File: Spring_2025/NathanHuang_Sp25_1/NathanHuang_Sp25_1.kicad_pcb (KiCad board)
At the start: 2 copper layers, 13 parts, among them J1 Barrel_Jack, M1 Motor_Servo, M2 Motor_Servo, M3 Motor_Servo, M4 Motor_Servo, M5 Motor_Servo, M6 Motor_Servo, M7 Stepper_Motor_bipolar, U1 ESP32-DEVKITC-32UE, U2 LM2596_BUCK_CONVERTER

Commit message: PCB Changes
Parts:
- removed the J1 at (240.5, 53.5)
- removed the J1 at (274.5, 48.0)
- added J1: Barrel_Jack, Connector_BarrelJack:BarrelJack_SwitchcraftConxall_RAPC10U_Horizontal, F.Cu at (54.7, 41.5)
- moved C1 178.3 mm to (74.0, 41.0), turned to 180 degrees
- moved A1 171.6 mm to (57.2, 93.2), turned to 180 degrees
- moved M7 160.1 mm to (76.5, 86.0), turned to 180 degrees
- moved U2 156.0 mm to (123.1, 49.0), turned to 180 degrees
- moved U1 52.4 mm to (103.2, 95.9)
- moved M6 27.6 mm to (143.5, 119.5)
- moved M5 26.7 mm to (143.6, 110.5)
- moved M4 24.4 mm to (143.1, 100.0)
- moved M3 23.0 mm to (143.0, 89.5)
- moved M2 21.5 mm to (143.1, 76.5)
- moved M1 21.2 mm to (143.0, 64.0)
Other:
- board outline added: 139.5 x 109.5 mm
- board text added: "12 V Side"
- board text added: "7.2 V Side"

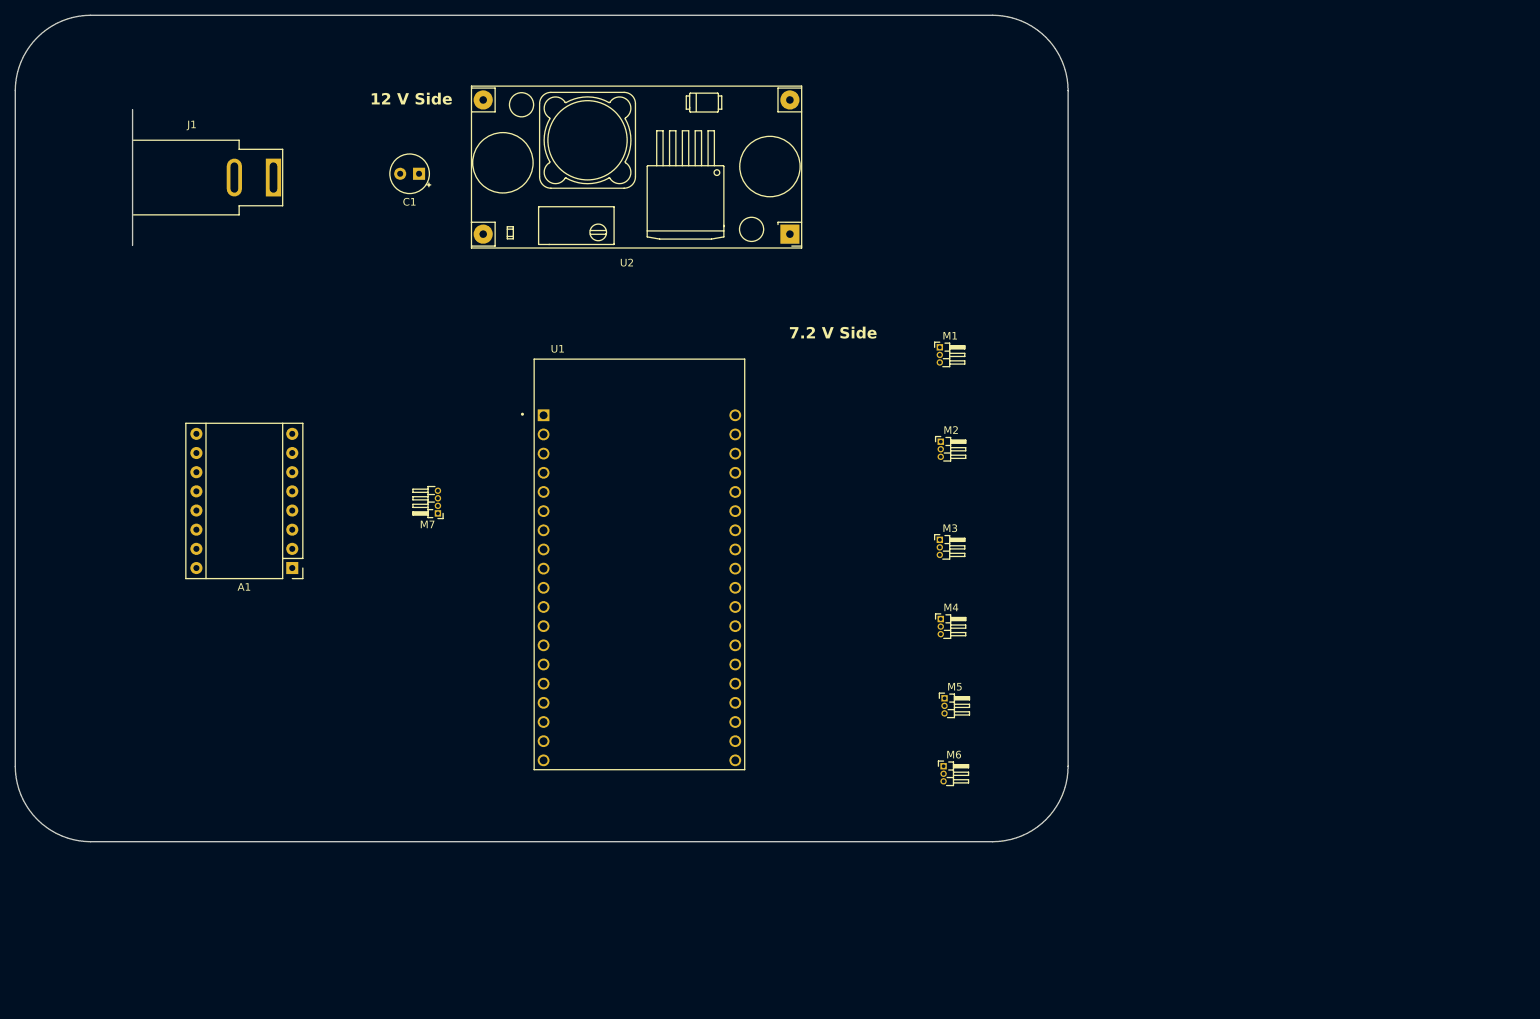
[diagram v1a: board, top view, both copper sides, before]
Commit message: Finished PCB, Ready for Print
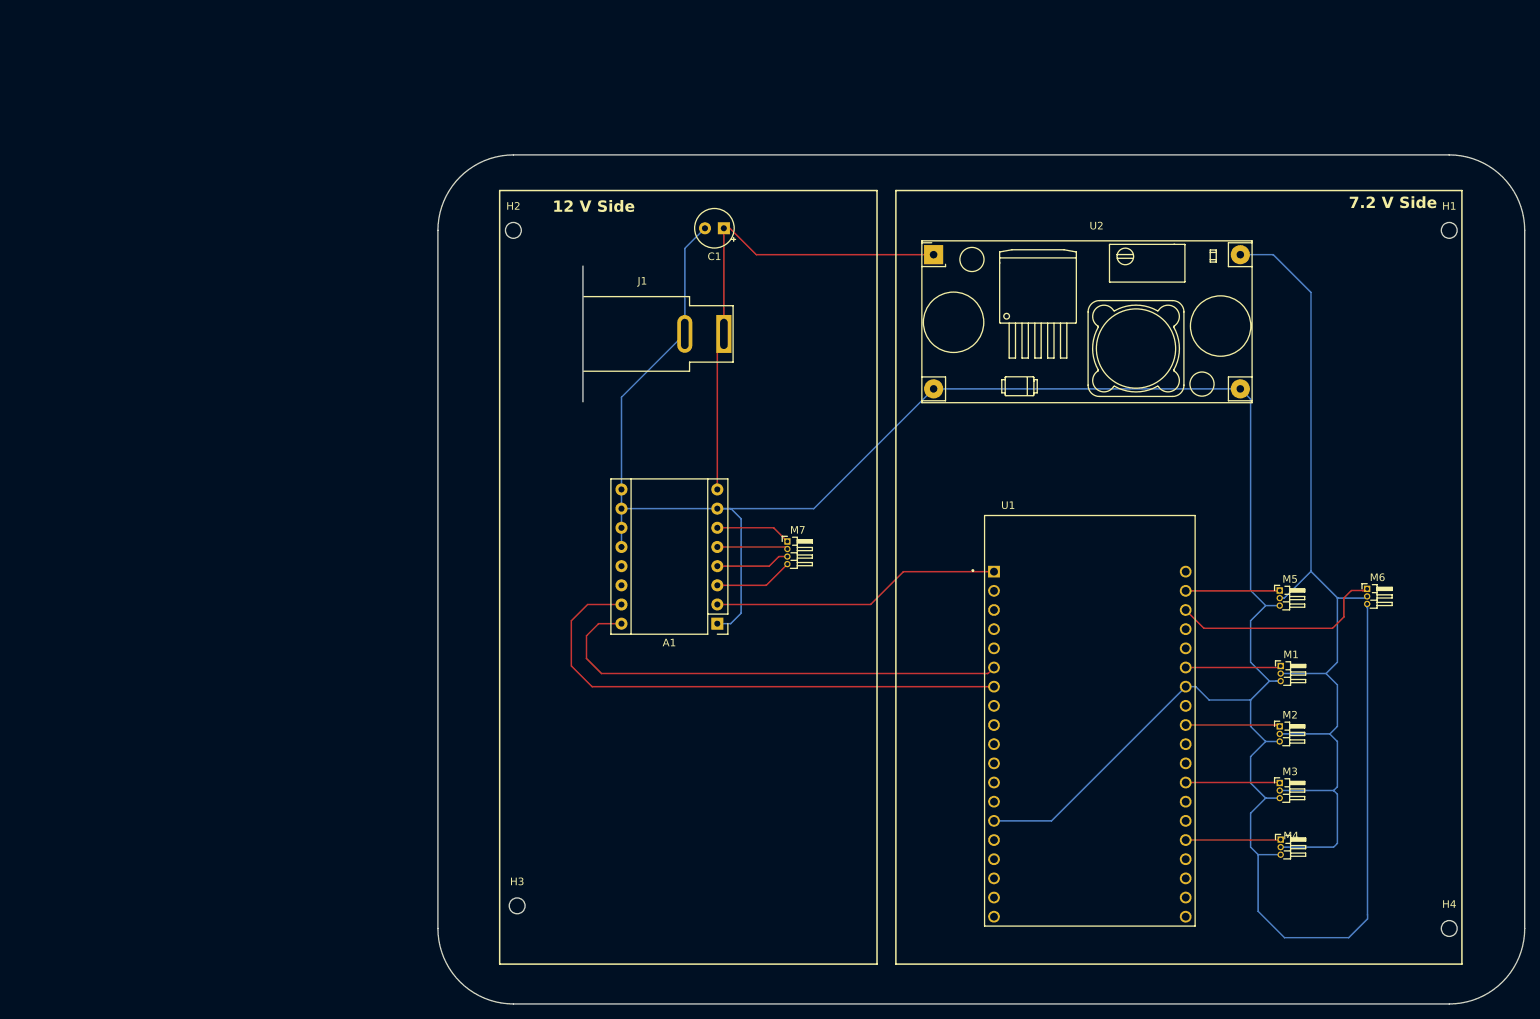
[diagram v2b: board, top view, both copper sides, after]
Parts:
- added H1: MountingHole, MountingHole:MountingHole_2.1mm, F.Cu at (210.5, 48.5)
- added H2: MountingHole, MountingHole:MountingHole_2.1mm, F.Cu at (86.5, 48.5)
- added H3: MountingHole, MountingHole:MountingHole_2.1mm, F.Cu at (87.0, 138.0)
- added H4: MountingHole, MountingHole:MountingHole_2.1mm, F.Cu at (210.5, 141.0)
- moved J1 63.2 mm to (114.4, 62.2)
- moved U1 63.2 mm to (162.9, 116.6)
- moved M1 61.8 mm to (188.2, 106.2)
- moved M6 60.8 mm to (199.6, 96.0)
- moved M2 58.7 mm to (188.0, 114.2)
- moved A1 56.8 mm to (113.5, 100.6)
- moved M3 55.4 mm to (188.0, 121.7)
- moved M4 53.7 mm to (188.2, 129.2)
- moved M5 46.7 mm to (188.0, 96.2)
- moved M7 46.5 mm to (122.8, 89.7), turned to 0 degrees
- moved C1 41.0 mm to (114.4, 48.2)
- moved U2 19.2 mm to (142.2, 51.7), turned to 0 degrees
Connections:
- A1 pad 2: +5V -> +3V3
- M7 pad 1: Net-(A1-1B) -> Net-(A1-2B)
- M7 pad 2: Net-(A1-1A) -> Net-(A1-2A)
- M7 pad 3: Net-(A1-2A) -> Net-(A1-1A)
- M7 pad 4: Net-(A1-2B) -> Net-(A1-1B)
- U1 pad 1: unconnected-(U1-3V3-Pad1) -> +3V3
- U1 pad 12: /STEP_PIN -> unconnected-(U1-14-Pad12)
- U1 pad 13: /THUMB_1 -> unconnected-(U1-12-Pad13)
- U1 pad 15: /THUMB_2 -> unconnected-(U1-13-Pad15)
- U1 pad 19: +5V -> unconnected-(U1-5V-Pad19)
- U1 pad 21: unconnected-(U1-23-Pad21) -> /THUMB_1
- U1 pad 22: unconnected-(U1-Pad22) -> /THUMB_2
- U1 pad 25: unconnected-(U1-21-Pad25) -> /INDEX
- U1 pad 28: unconnected-(U1-18-Pad28) -> /MIDDLE
- U1 pad 29: /PINKIE -> unconnected-(U1-5-Pad29)
- U1 pad 31: unconnected-(U1-16-Pad31) -> /RING
- U1 pad 32: /RING -> unconnected-(U1-4-Pad32)
- U1 pad 33: /INDEX -> unconnected-(U1-0-Pad33)
- U1 pad 34: /MIDDLE -> /PINKIE
- U1 pad 35: /DIR_PIN -> unconnected-(U1-15-Pad35)
- U1 pad 6: unconnected-(U1-35-Pad6) -> /DIR_PIN
- U1 pad 7: unconnected-(U1-32-Pad7) -> /STEP_PIN
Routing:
- net GND: track 0.00 -> 344.3 mm
- net 7.2V: track 0.00 -> 125.7 mm
- net /STEP_PIN: track 0.00 -> 70.7 mm
- net +12V: track 0.00 -> 64.2 mm
- net /DIR_PIN: track 0.00 -> 63.5 mm
- net +3V3: track 0.00 -> 38.5 mm
- net /THUMB_2: track 0.00 -> 29.3 mm
- net /INDEX: track 0.00 -> 12.7 mm
- net /PINKIE: track 0.00 -> 12.6 mm
- net /MIDDLE: track 0.00 -> 12.5 mm
- net /RING: track 0.00 -> 12.5 mm
- net /THUMB_1: track 0.00 -> 12.5 mm
- net Net-(A1-1B): track 0.00 -> 10.4 mm
- net Net-(A1-2B): track 0.00 -> 10.0 mm
- net Net-(A1-1A): track 0.00 -> 9.81 mm
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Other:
- board size 139.5 x 109.5 mm -> 144 x 112.5 mm

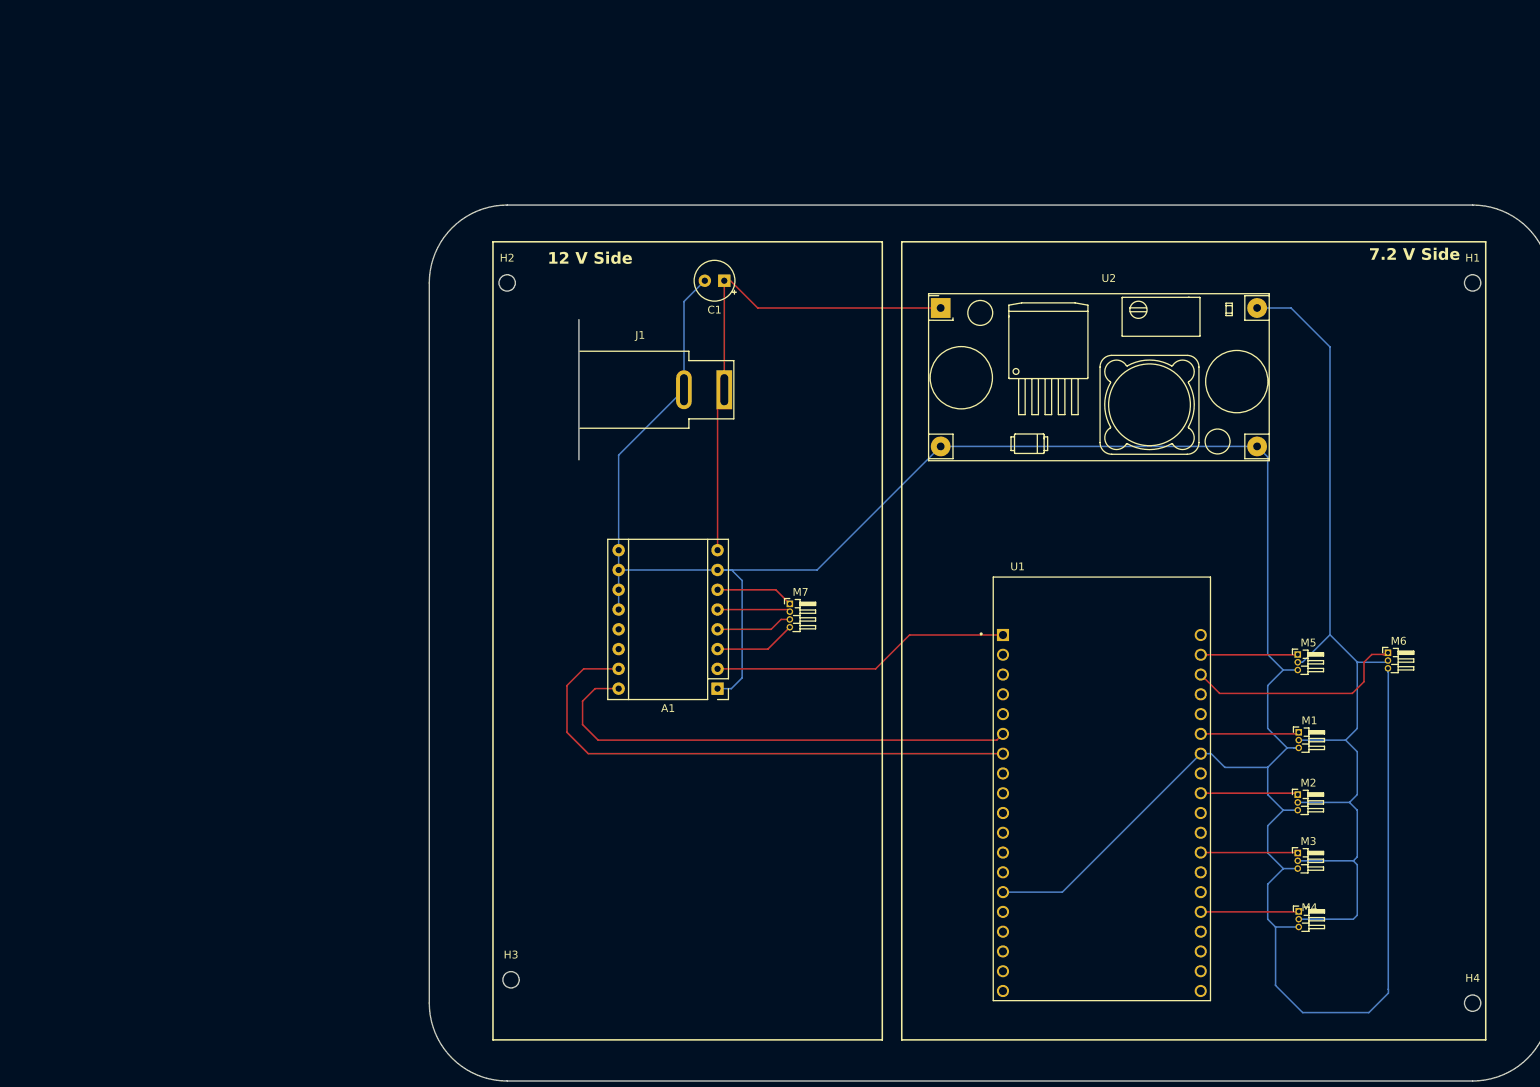
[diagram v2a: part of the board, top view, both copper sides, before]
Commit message: PCB Updates
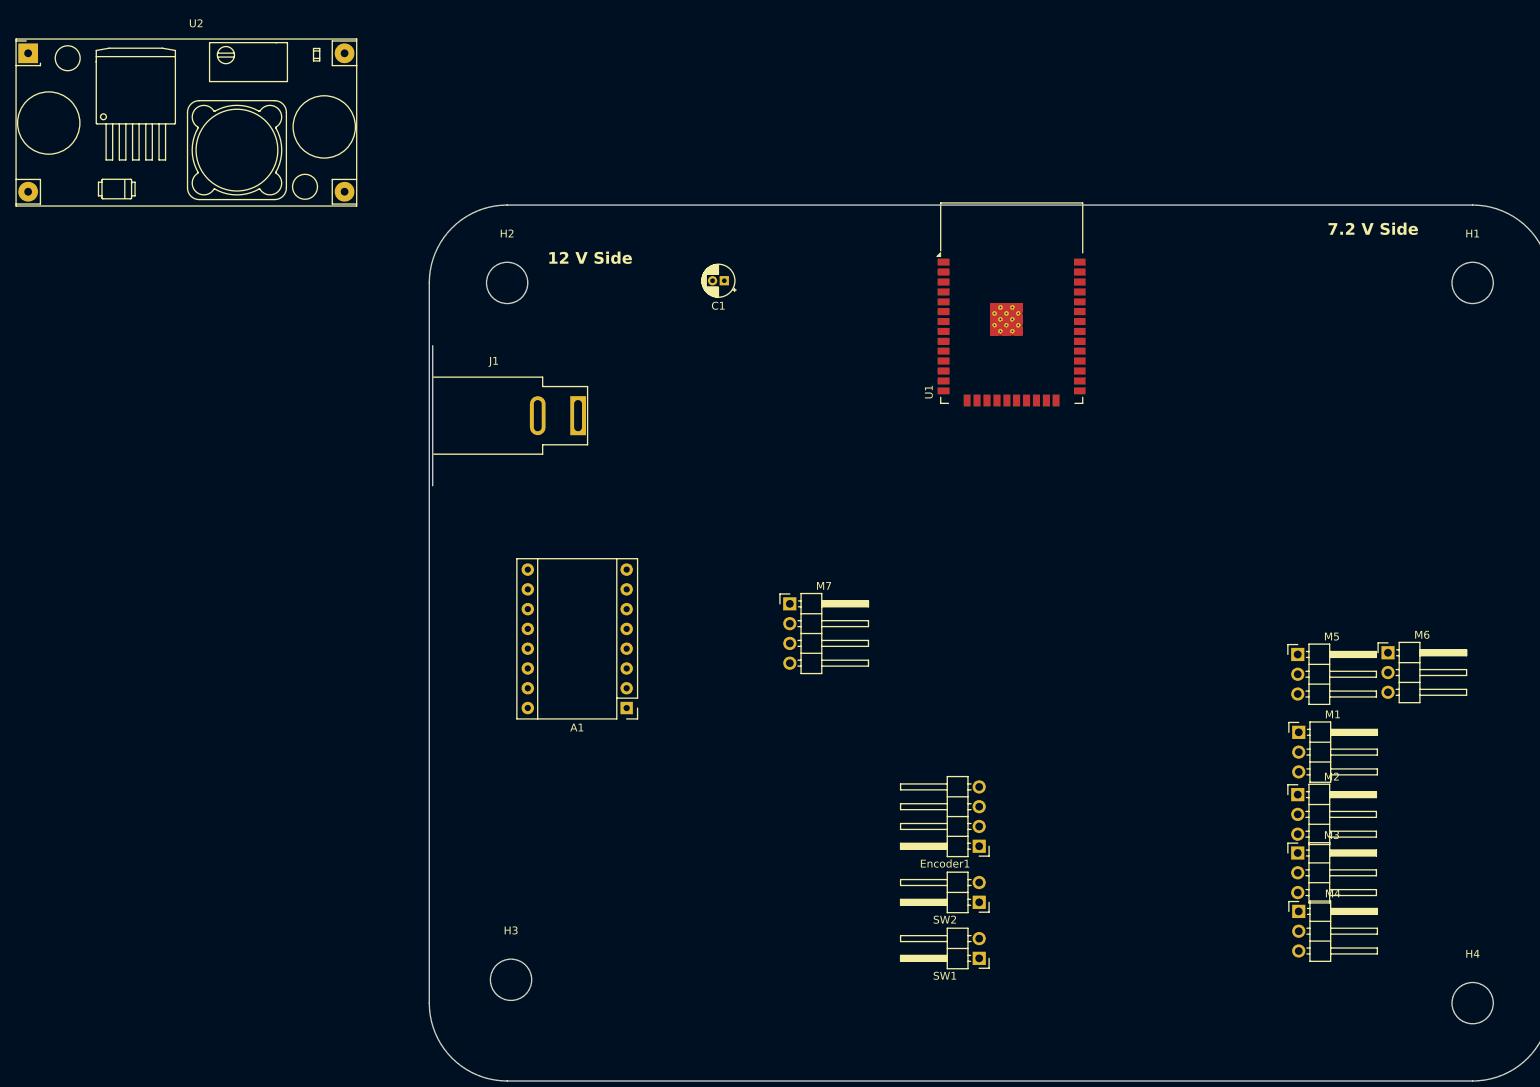
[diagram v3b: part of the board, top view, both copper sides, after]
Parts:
- added Encoder1: ~, Connector_PinHeader_2.54mm:PinHeader_1x04_P2.54mm_Horizontal, F.Cu at (147.1, 120.8)
- added SW1: SW_Push, Connector_PinHeader_2.54mm:PinHeader_1x02_P2.54mm_Horizontal, F.Cu at (147.1, 135.2)
- added SW2: SW_Push, Connector_PinHeader_2.54mm:PinHeader_1x02_P2.54mm_Horizontal, F.Cu at (147.1, 128.1)
- C1: footprint Capacitor_THT:CP_Radial_Tantal_D5.0mm_P2.50mm -> Capacitor_THT:CP_Radial_D4.0mm_P1.50mm
- H1, H2, H3, H4: footprint MountingHole:MountingHole_2.1mm -> MountingHole:MountingHole_5.3mm_M5
- M1, M2, M3, M4, M5, M6: footprint Connector_PinHeader_1.00mm:PinHeader_1x03_P1.00mm_Horizontal -> Connector_PinHeader_2.54mm:PinHeader_1x03_P2.54mm_Horizontal
- M7: footprint Connector_PinHeader_1.00mm:PinHeader_1x04_P1.00mm_Horizontal -> Connector_PinHeader_2.54mm:PinHeader_1x04_P2.54mm_Horizontal
- U1: value ESP32-DEVKITC-32UE -> ESP32-WROOM-32; footprint Library:ESP32-DEVKITC-32UE -> RF_Module:ESP32-WROOM-32
- moved U2 121.7 mm to (25.0, 19.0)
- moved U1 63.6 mm to (151.3, 54.1)
- moved J1 19.1 mm to (95.6, 65.5)
- moved A1 11.9 mm to (101.8, 103.1)
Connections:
- U1 pad 1: +3V3 -> GND
- U1 pad 13: unconnected-(U1-12-Pad13) -> /DT
- U1 pad 14: GND -> /PINKIE
- U1 pad 15: unconnected-(U1-13-Pad15) -> GND
- U1 pad 16: unconnected-(U1-D2-Pad16) -> /CW
- U1 pad 2: unconnected-(U1-EN-Pad2) -> +3V3
- U1 pad 21: /THUMB_1 -> unconnected-(U1-SDO/SD0-Pad21)
- U1 pad 22: /THUMB_2 -> unconnected-(U1-SDI/SD1-Pad22)
- U1 pad 23: unconnected-(U1-TX-Pad23) -> /RING
- U1 pad 25: /INDEX -> Net-(U1-IO0)
- U1 pad 26: GND -> Net-(U1-IO4)
- U1 pad 27: unconnected-(U1-19-Pad27) -> /MIDDLE
- U1 pad 28: /MIDDLE -> /INDEX
- U1 pad 30: unconnected-(U1-17-Pad30) -> /THUMB_2
- U1 pad 31: /RING -> /THUMB_1
- U1 pad 33: unconnected-(U1-0-Pad33) -> /STEP_PIN
- U1 pad 34: /PINKIE -> unconnected-(U1-RXD0/IO3-Pad34)
- U1 pad 36: unconnected-(U1-D1-Pad36) -> /DIR_PIN
- U1 pad 38: unconnected-(U1-CLK-Pad38) -> GND
- U1 pad 6: /DIR_PIN -> unconnected-(U1-IO34-Pad6)
- U1 pad 7: /STEP_PIN -> unconnected-(U1-IO35-Pad7)
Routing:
- net GND: track 344.3 -> 0.00 mm
- net 7.2V: track 125.7 -> 0.00 mm
- net /STEP_PIN: track 70.7 -> 0.00 mm
- net +12V: track 64.2 -> 0.00 mm
- net /DIR_PIN: track 63.5 -> 0.00 mm
- net +3V3: track 38.5 -> 0.00 mm
- net /THUMB_2: track 29.3 -> 0.00 mm
- net /INDEX: track 12.7 -> 0.00 mm
- net /PINKIE: track 12.6 -> 0.00 mm
- net /MIDDLE: track 12.5 -> 0.00 mm
- net /RING: track 12.5 -> 0.00 mm
- net /THUMB_1: track 12.5 -> 0.00 mm
- net Net-(A1-1B): track 10.4 -> 0.00 mm
- net Net-(A1-2B): track 10.0 -> 0.00 mm
- net Net-(A1-1A): track 9.81 -> 0.00 mm
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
